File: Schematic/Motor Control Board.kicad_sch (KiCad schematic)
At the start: 0 parts

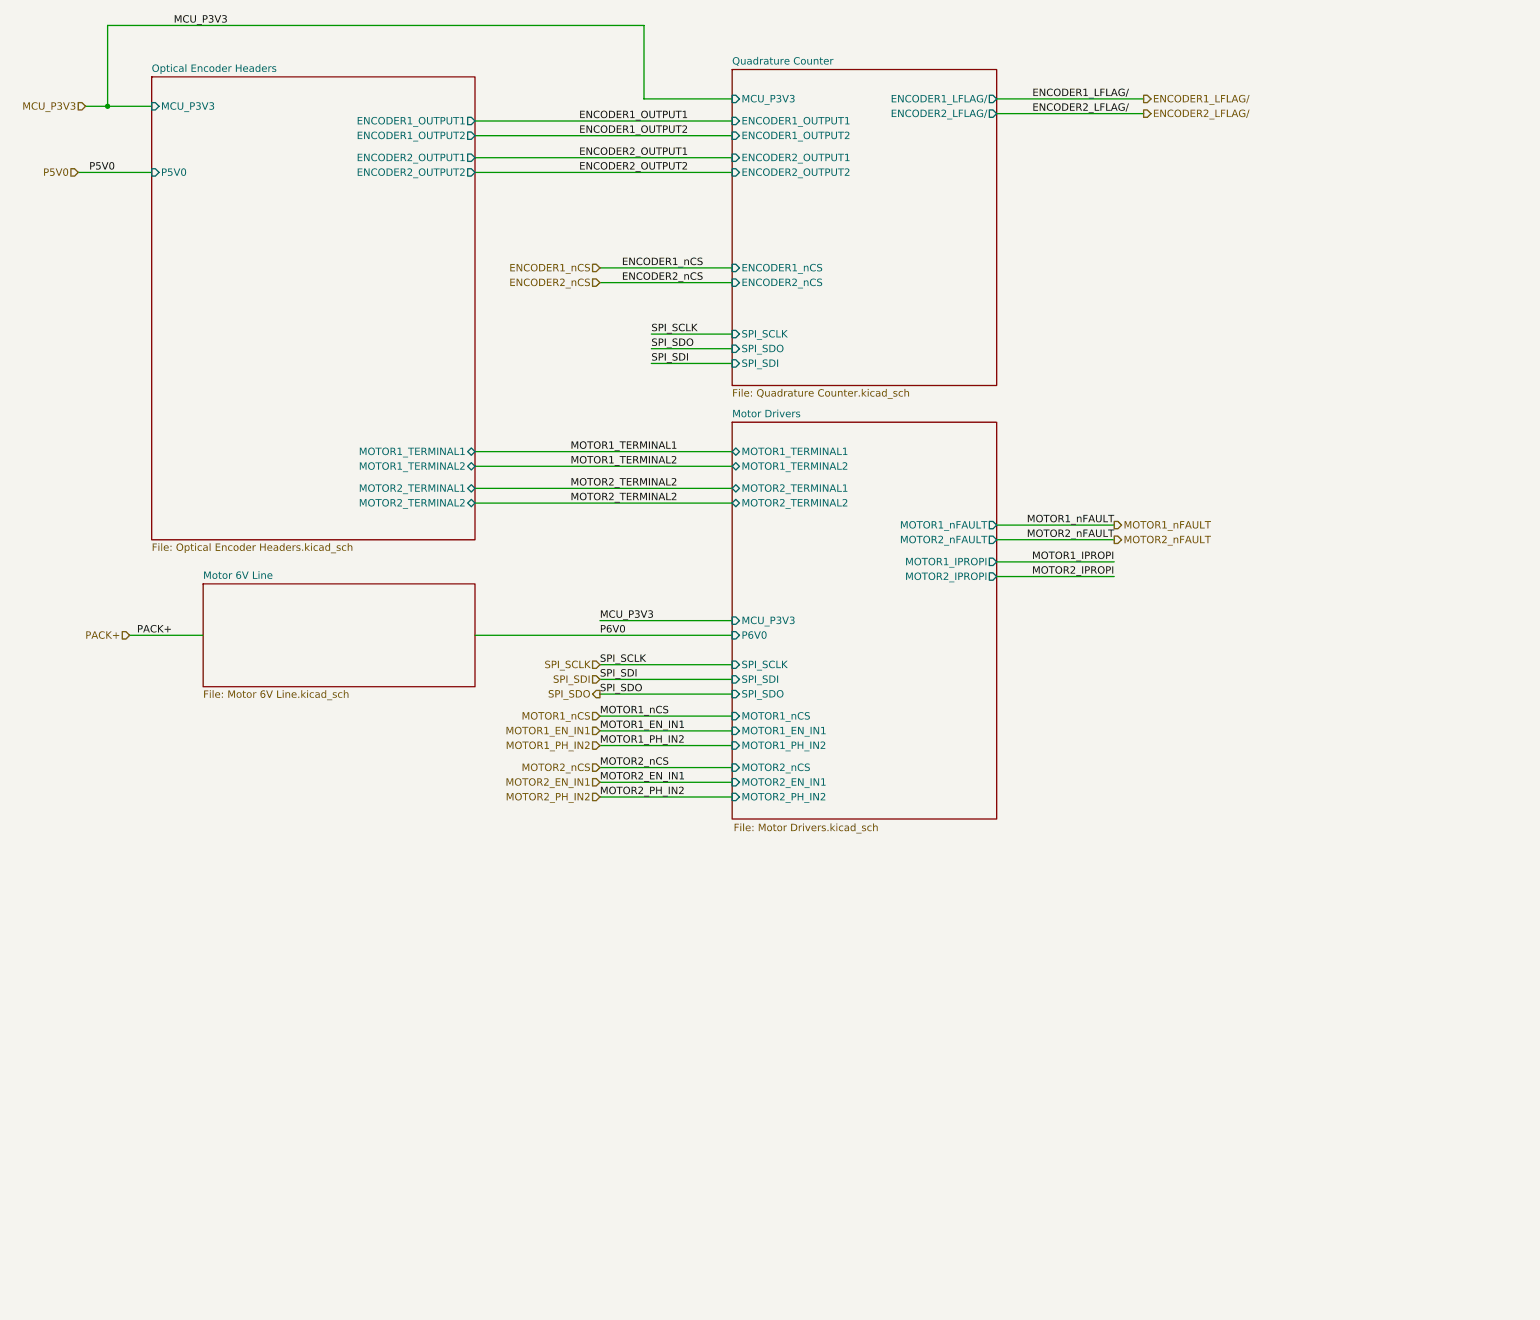
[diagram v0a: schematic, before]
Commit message: updated
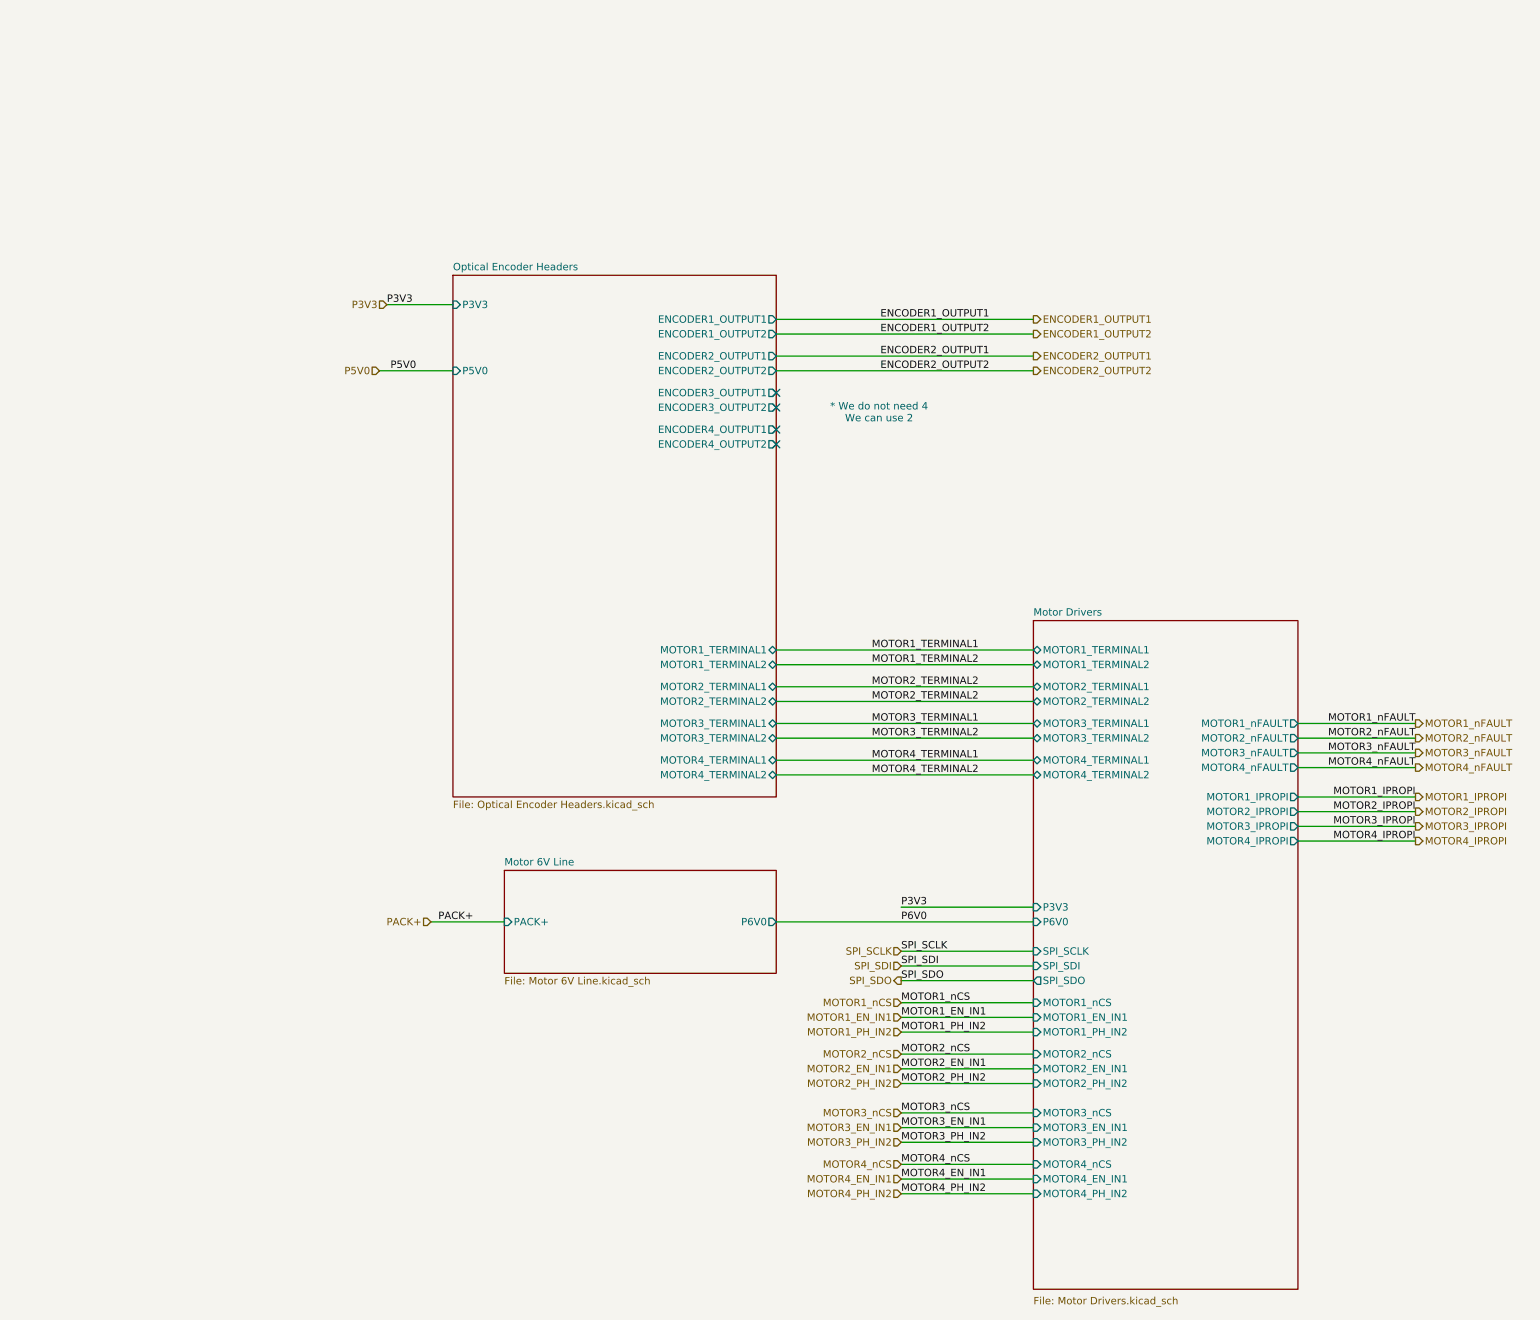
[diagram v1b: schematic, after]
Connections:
- no-connect marks 0 -> 4
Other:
- removed sheet Quadrature Counter
- sheet Motor 6V Line ports: added P6V0, PACK+; removed none
- sheet Motor Drivers ports: added MOTOR3_EN_IN1, MOTOR3_IPROPI, MOTOR3_PH_IN2, MOTOR3_TERMINAL1, MOTOR3_TERMINAL2, MOTOR3_nCS, MOTOR3_nFAULT, MOTOR4_EN_IN1, MOTOR4_IPROPI, MOTOR4_PH_IN2, MOTOR4_TERMINAL1, MOTOR4_TERMINAL2, MOTOR4_nCS, MOTOR4_nFAULT, P3V3; removed MCU_P3V3
- sheet Optical Encoder Headers ports: added ENCODER3_OUTPUT1, ENCODER3_OUTPUT2, ENCODER4_OUTPUT1, ENCODER4_OUTPUT2, MOTOR3_TERMINAL1, MOTOR3_TERMINAL2, MOTOR4_TERMINAL1, MOTOR4_TERMINAL2, P3V3; removed MCU_P3V3
- note added: "* We do not need 4 We can use 2"
